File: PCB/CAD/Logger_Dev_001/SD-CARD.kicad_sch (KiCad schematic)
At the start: 1 part, among them J1 Micro_SD_Card_Det2

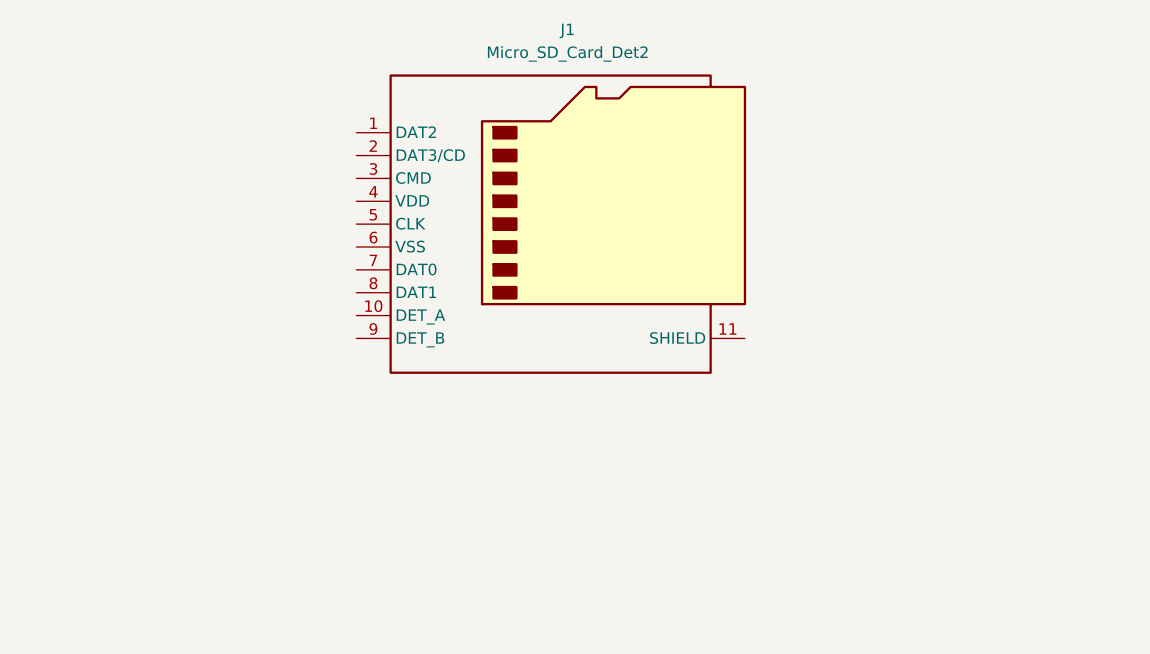
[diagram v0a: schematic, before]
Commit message: Library Submodule Update
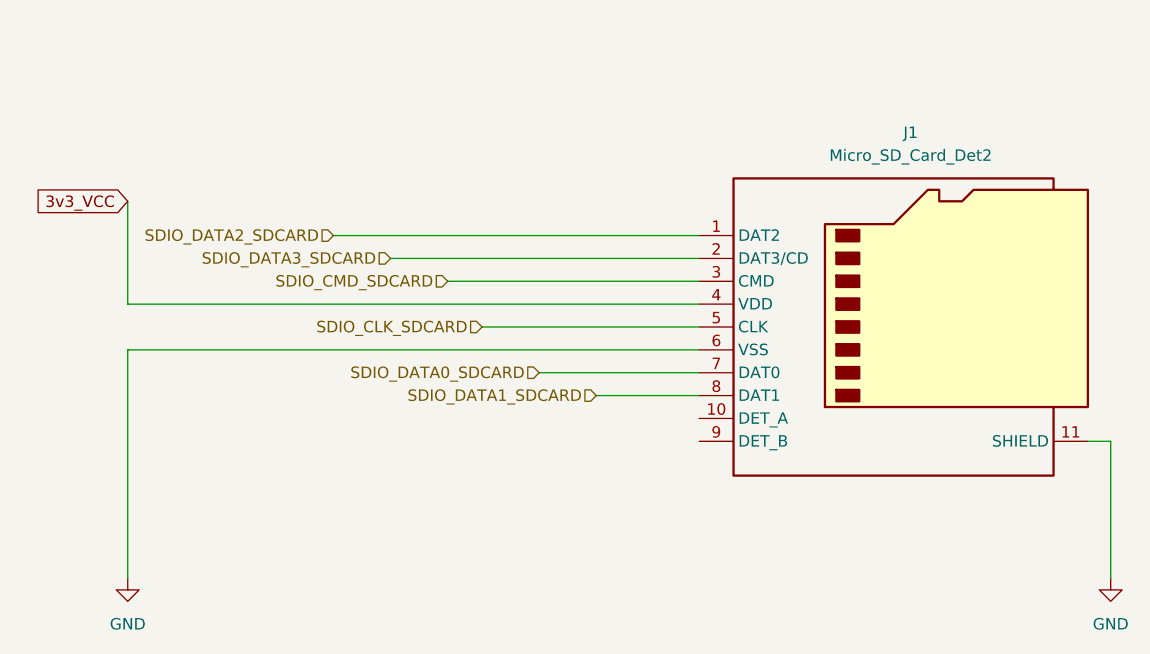
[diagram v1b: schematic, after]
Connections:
- net SDIO_DATA2_SDCARD: now reaches J1.1 (DAT2)
- net GND: now reaches J1.11 (SHIELD)
- net GND: now also J1.6 (VSS)
- net SDIO_DATA3_SDCARD: now reaches J1.2 (DAT3/CD)
- net SDIO_CMD_SDCARD: now reaches J1.3 (CMD)
- net 3v3_VCC: now reaches J1.4 (VDD)
- net SDIO_CLK_SDCARD: now reaches J1.5 (CLK)
- net SDIO_DATA0_SDCARD: now reaches J1.7 (DAT0)
- net SDIO_DATA1_SDCARD: now reaches J1.8 (DAT1)
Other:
- moved on the sheet: J1
